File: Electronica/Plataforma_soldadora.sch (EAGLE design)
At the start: 26 parts, among them J1 22-27-2021-02, SW2 ROTARTY_ENCODER, T1 BTA06400B, U1 RPDZN5W6H, U5 ESP32-C3_SUPERMINISMD

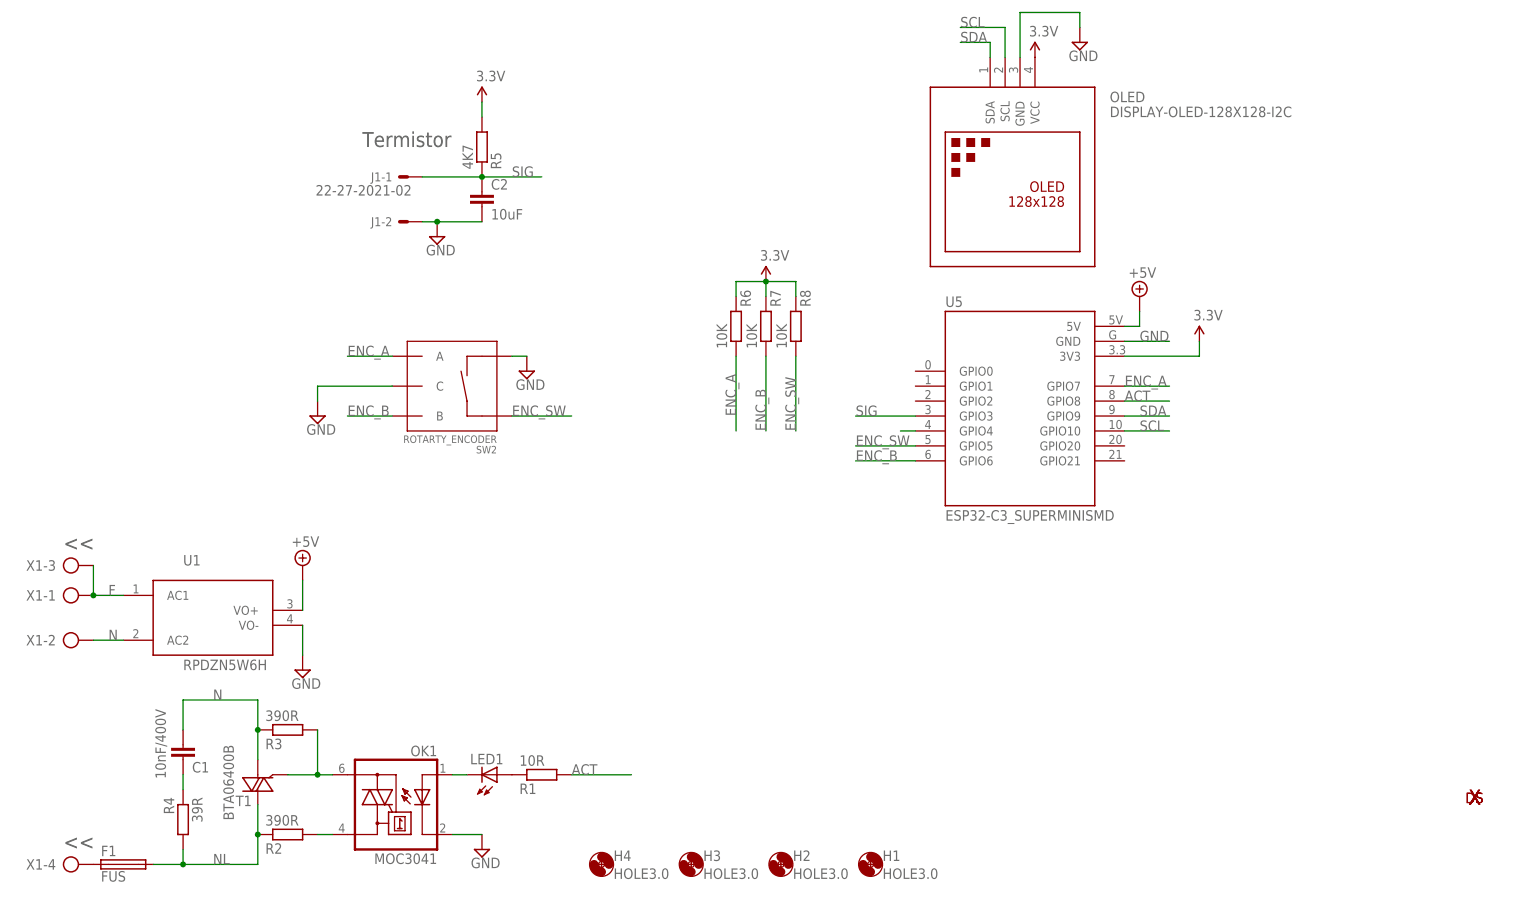
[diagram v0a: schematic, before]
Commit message: Update
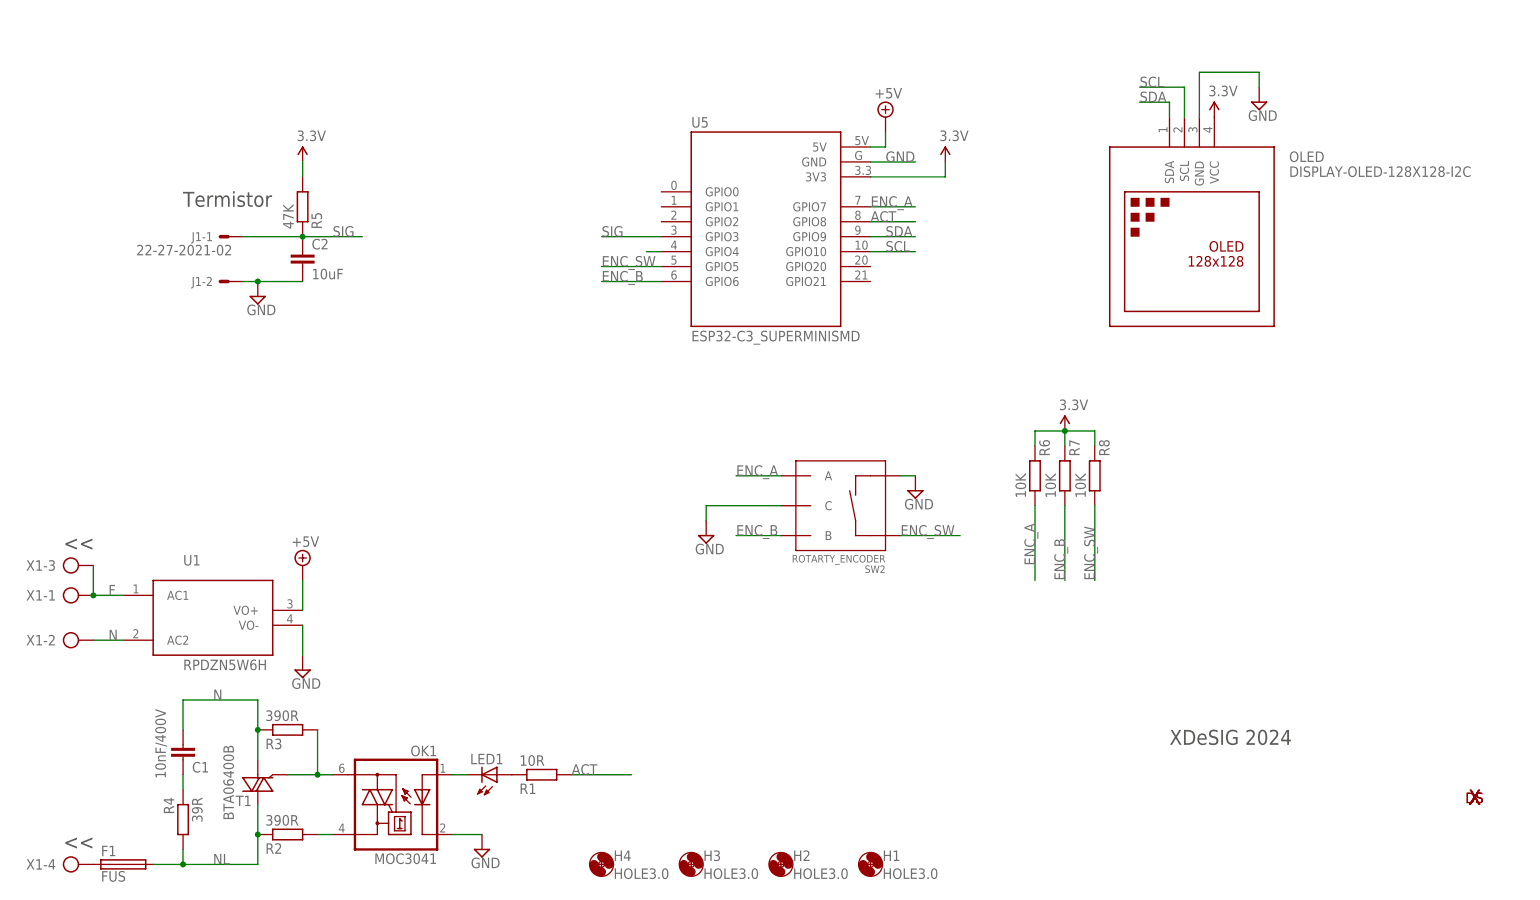
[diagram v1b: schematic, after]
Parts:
- R5: value 4K7 -> 47K
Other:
- note added: "Uns capacitores de 100nF estarían ben"
- note added: "XDeSIG 2024"
- note removed: "cambiar a 47K"
- note removed: "por capacitores de 1uF no encoder"
- moved on the sheet: C2, J1-1, J1-2, OLED, R5, R6, R7, R8, SW2, U5
